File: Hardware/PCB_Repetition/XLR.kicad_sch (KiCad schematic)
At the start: 4 parts, among them J5 XLR3, J7 XLR3, SW3 SW_DIP_x02

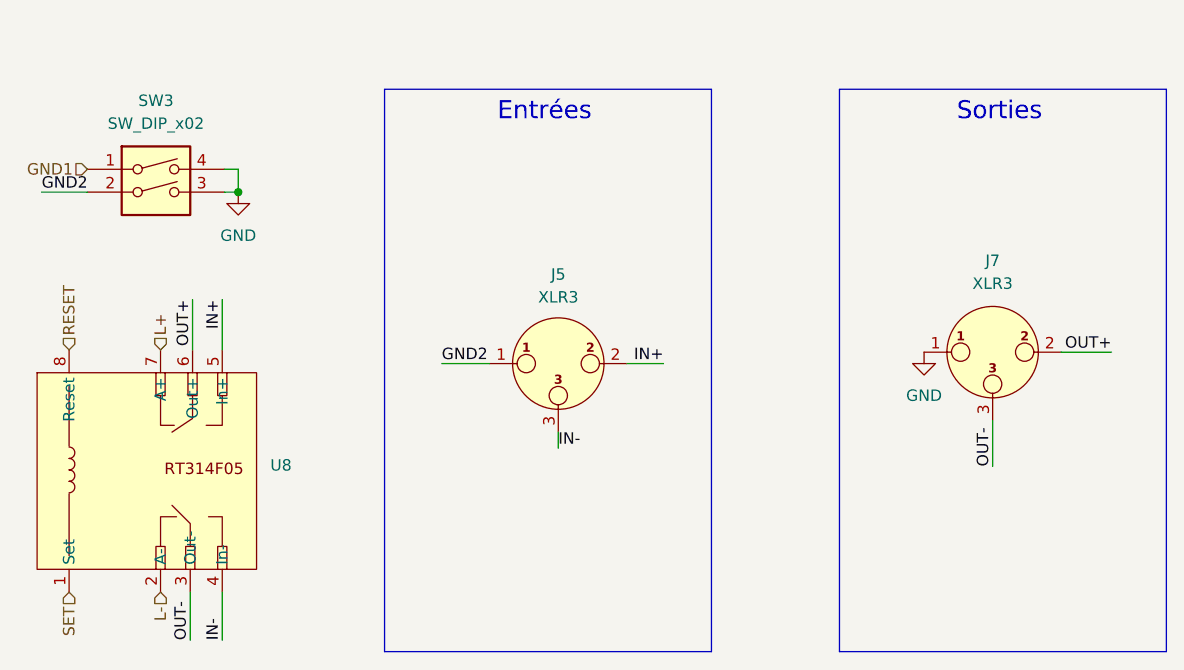
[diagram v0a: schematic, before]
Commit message: finalisation PCB-salle de Répétition
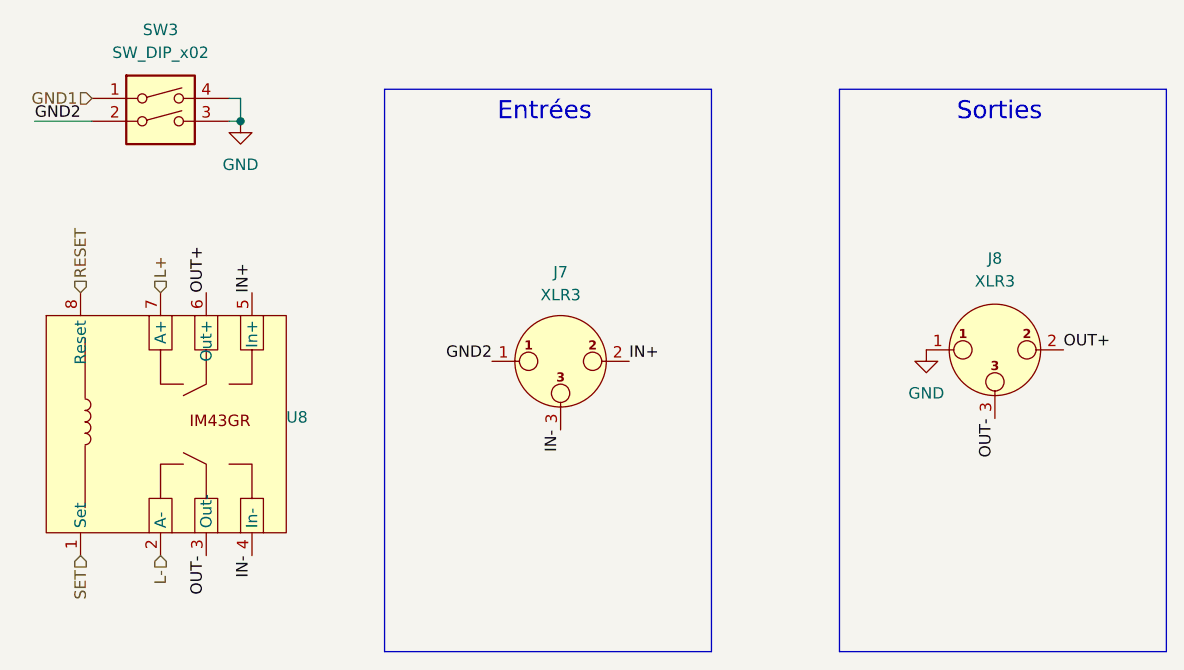
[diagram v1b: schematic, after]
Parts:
- U8: footprint (none) -> Relais_Sig:IM43GR
- renumbered J5 to J7, J7 to J8
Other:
- moved on the sheet: SW3, U8
